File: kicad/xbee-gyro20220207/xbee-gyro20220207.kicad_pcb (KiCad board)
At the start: 2 copper layers, 69.2 x 61.6 mm, 17 parts, among them J1 IMU_in, J2 IMU, J3 XBee, SW1 Reset, U1 XBEE-S2C, U2 XC6216D_SOT89

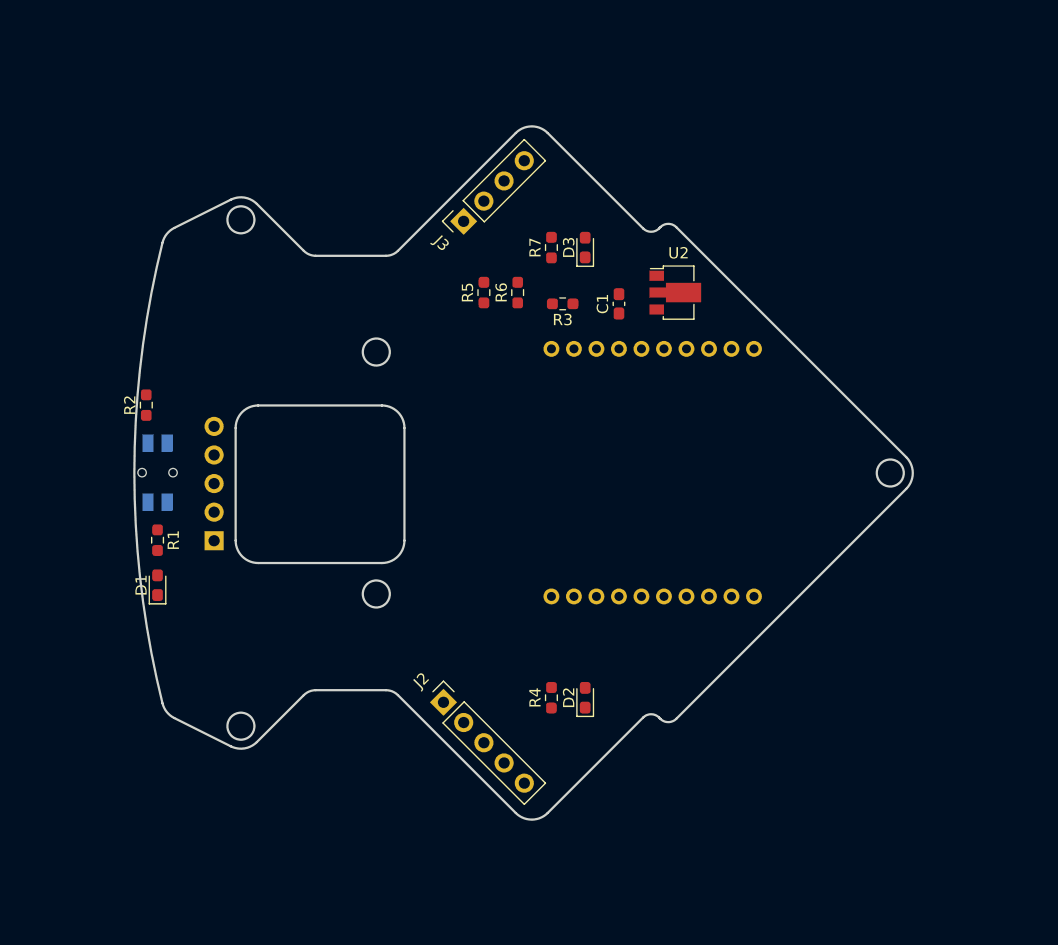
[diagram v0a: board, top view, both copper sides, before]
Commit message: iicad
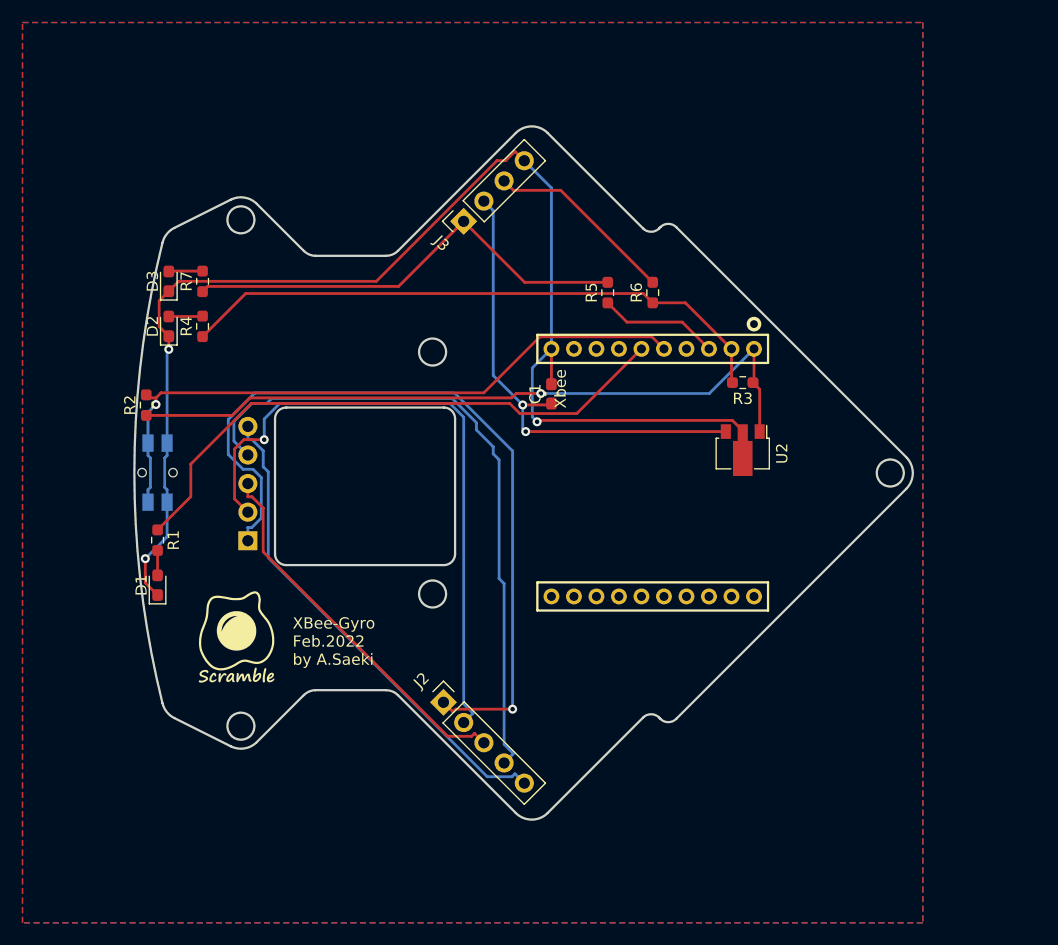
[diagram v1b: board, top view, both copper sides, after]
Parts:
- added G***: LOGO, LOGO, F.Cu at (54.0, 130.0)
- U1: moved to F.Cu
- moved D2 49.6 mm to (48.0, 102.0)
- moved R4 45.3 mm to (51.0, 102.0)
- moved D3 37.1 mm to (48.0, 98.0)
- moved R7 31.1 mm to (51.0, 98.0)
- moved R3 17.5 mm to (99.0, 107.0)
- moved U2 15.2 mm to (99.0, 113.0), turned to -90 degrees
- moved R6 12.0 mm to (91.0, 99.0)
- moved R5 11.0 mm to (87.0, 99.0)
- moved C1 10.0 mm to (82.0, 108.0)
- moved J1 3.00 mm to (55.0, 121.0)
- turned U1 to -90 degrees
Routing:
- net GND: track 0.00 -> 113.4 mm, vias 0 -> 3
- net Net-(J1-Pad1): track 0.00 -> 71.1 mm, vias 0 -> 1
- net Net-(R2-Pad1): track 0.00 -> 64.1 mm, vias 0 -> 1
- net Net-(J1-Pad4): track 0.00 -> 58.7 mm
- net Net-(R2-Pad2): track 0.00 -> 58.5 mm, vias 0 -> 1
- net Net-(J1-Pad2): track 0.00 -> 57.5 mm, vias 0 -> 1
- net Net-(R3-Pad2): track 0.00 -> 53.7 mm
- net Net-(R1-Pad1): track 0.00 -> 52.1 mm
- net Net-(J1-Pad5): track 0.00 -> 43.9 mm
- net +5V: track 0.00 -> 42.4 mm, vias 0 -> 2
- net Net-(J3-Pad1): track 0.00 -> 40.8 mm
- net Net-(J1-Pad3): track 0.00 -> 33.7 mm
- net Net-(J3-Pad3): track 0.00 -> 16.9 mm
- net Net-(R5-Pad1): track 0.00 -> 10.7 mm
- net Net-(D3-Pad2): track 0.00 -> 3.02 mm
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- added copper zone on B.Cu, net GND
- added copper zone on F.Cu, net GND
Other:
- outline, holes or cut-outs redrawn
- board text added: "XBee-Gyro Feb.2022 by A.Saeki"

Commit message: no message
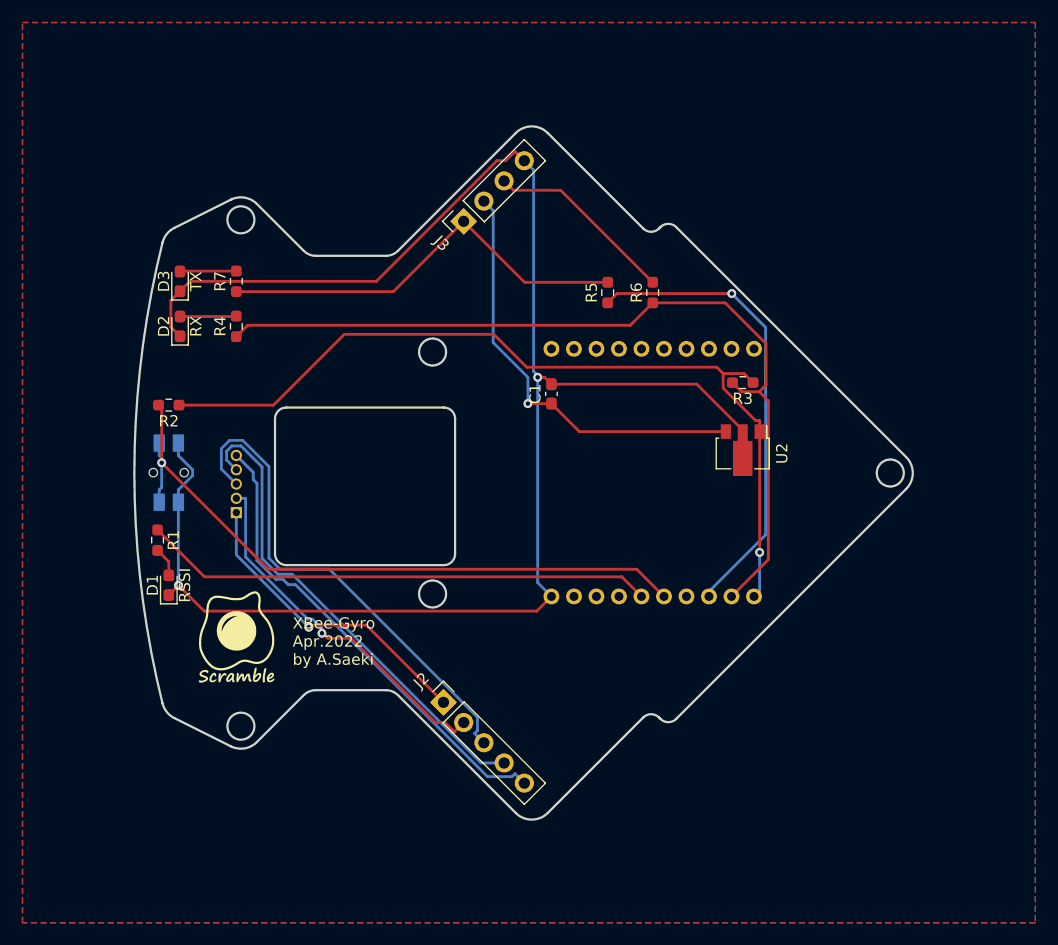
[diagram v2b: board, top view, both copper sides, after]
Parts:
- J1: footprint Connector_PinSocket_2.54mm:PinSocket_1x05_P2.54mm_Vertical -> Connector_PinHeader_1.27mm:PinHeader_1x05_P1.27mm_Vertical
- U1: moved to B.Cu
- moved R4 3.00 mm to (54.0, 102.0)
- moved R7 3.00 mm to (54.0, 98.0)
- moved J1 2.70 mm to (54.0, 118.5)
- moved R2 2.00 mm to (48.0, 109.0), turned to 180 degrees
- moved D1 1.00 mm to (48.0, 125.0)
- moved D2 1.00 mm to (49.0, 102.0)
- moved D3 1.00 mm to (49.0, 98.0)
- moved SW1 1.00 mm to (48.0, 115.0)
- turned U1 to 90 degrees
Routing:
- net Net-(J1-Pad1): track 71.1 -> 27.7 mm
- net GND: track 113.4 -> 150.4 mm, vias 3 -> 2
- net Net-(R5-Pad1): track 10.7 -> 41.6 mm, vias 0 -> 1
- net Net-(J1-Pad2): track 57.5 -> 32.4 mm
- net Net-(R3-Pad2): track 53.7 -> 76.9 mm
- net Net-(J1-Pad4): track 58.7 -> 43.3 mm
- net Net-(R2-Pad1): track 64.1 -> 76.9 mm
- net Net-(J1-Pad3): track 33.7 -> 44.4 mm
- net Net-(R1-Pad1): track 52.1 -> 45.4 mm
- net +5V: track 42.4 -> 38.2 mm, vias 2 -> 1
- net Net-(J3-Pad1): track 40.8 -> 37.8 mm
- net Net-(D3-Pad2): track 3.02 -> 5.02 mm
- net Net-(D2-Pad2): track 3.02 -> 5.02 mm
- net Net-(R2-Pad2): track 58.5 -> 60.2 mm
- net Net-(J1-Pad5): track 43.9 -> 42.3 mm
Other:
- board text added: "XBee-Gyro Apr.2022 by A.Saeki"
- board text removed: "XBee-Gyro Feb.2022 by A.Saeki"
